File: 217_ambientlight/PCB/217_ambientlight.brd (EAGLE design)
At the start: 27.9 x 39.4 mm, 10 parts, among them IC2 IN-ISL29034

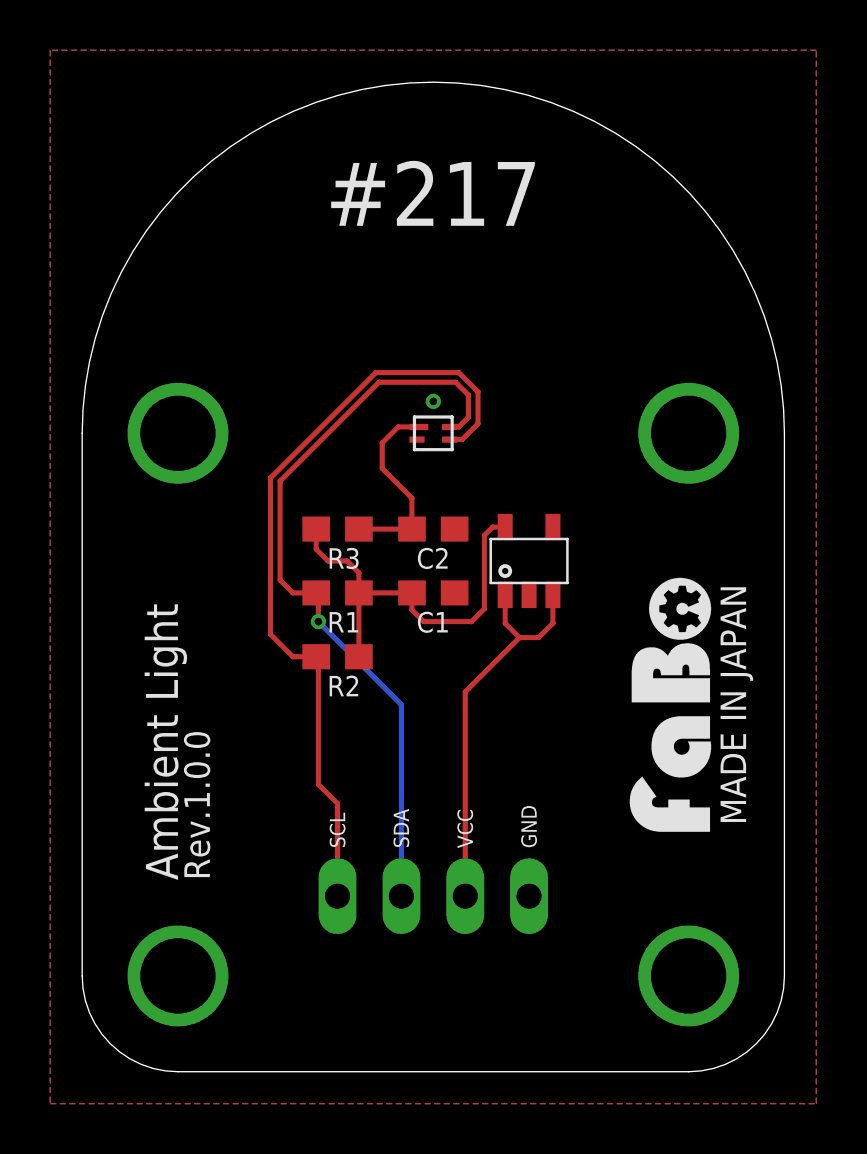
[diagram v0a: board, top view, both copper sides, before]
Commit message: change dru seeed
212 is draft
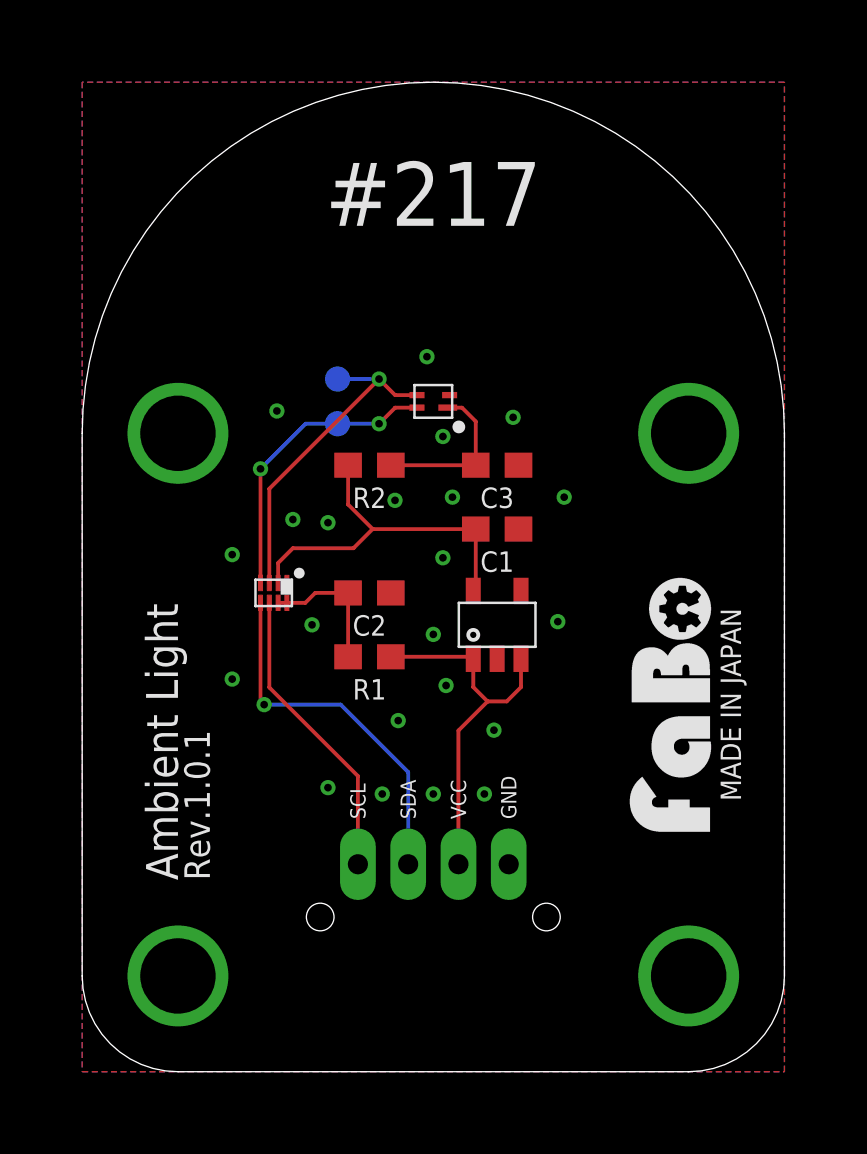
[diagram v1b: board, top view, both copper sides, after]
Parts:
- removed R3: 100, FaBo-Resistors:0603
- added C3: 1uF, FaBo-Capacitor:0603
- added IC3: (no value), FaBo-Mems:INTERSIL-ISL29034
- added TP1, TP2: (no value), FaBo-Supply:TP-10
- C2: value 1uF -> 0.1uF
- IC2: value IN-ISL29034 -> (none); device FaBo-Mems:INTERSIL-ISL29034 -> FaBo-LevelTranslator:X2SON
- R1: value 4.7k -> 200k
- R2: value 4.7k -> 100
- U$2: device FaBo-etc:LOGO_OSHW_T_MS_BOTTOM -> FaBo-etc:LOGO_OSHW_M_BOTTOM
- moved IC2 8.98 mm to (7.62, 19.1), turned to 180 degrees
- moved R2 7.73 mm to (11.4, 24.1), turned to 180 degrees
- moved C1 3.59 mm to (16.5, 21.6)
- moved C2 3.59 mm to (11.4, 19.1)
- moved IC1 2.84 mm to (16.5, 17.8)
- moved R1 2.84 mm to (11.4, 16.5)
- moved U$2 0.38 mm to (14.0, 3.17)
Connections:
- new net N$1: C2.2, IC2.7, IC2.8, R1.1
- new net SCL_HV: IC2.6, J1.SCL
- new net SDA_HV: IC2.5, J1.SDA
- net 3V3: now also IC2.2; no longer R1.2, R3.2
- net 5V: now also R1.2
- net GND: now also C3.1, IC2.1, IC3.2; no longer IC2.2
- net SCL: now also IC3.3, TP2.1; no longer J1.SCL, R2.1
- net SDA: now also IC3.4, TP1.1; no longer J1.SDA, R1.1
- net VCC: now also C3.2, IC3.1, R2.1; no longer C2.2, IC2.1, R3.1
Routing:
- net SDA: track 30.2 -> 11.8 mm, vias 1 -> 2
- net SCL: track 31.3 -> 13.3 mm, vias 0 -> 1
- net SDA_HV: track 0.00 -> 14.6 mm, vias 0 -> 1
- net SCL_HV: track 0.00 -> 11.9 mm
- net N$1: track 0.00 -> 5.49 mm
- net 3V3: track 16.2 -> 14.7 mm
- net VCC: track 7.75 -> 6.46 mm
- net 5V: track 15.8 -> 14.9 mm
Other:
- board text added: "Rev.1.0.1"
- board text removed: "Rev.1.0.0"
